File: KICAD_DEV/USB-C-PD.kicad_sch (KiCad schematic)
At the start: 36 parts, among them J1 USB_C_Receptacle_USB2.0_14P, Q1 NMOS, U2 TPS26750, U3 TPD4S480

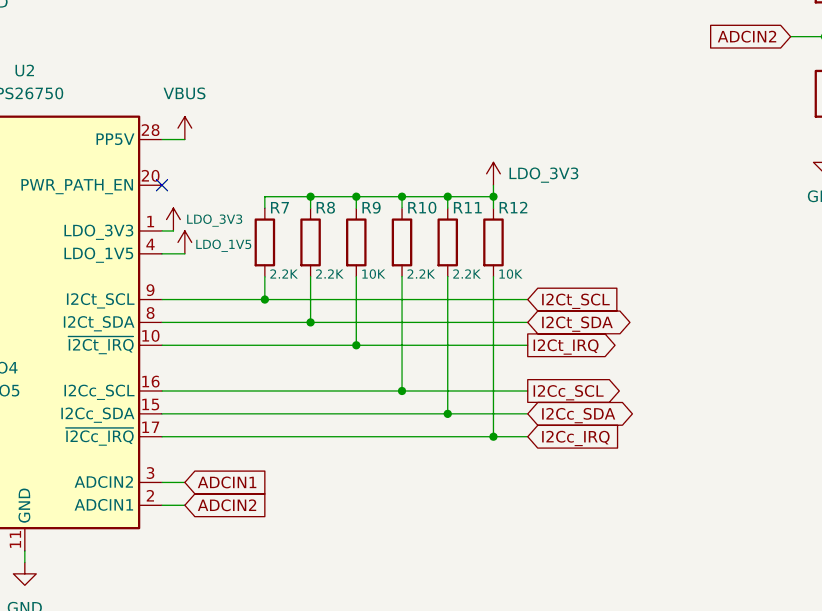
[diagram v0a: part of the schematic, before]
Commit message: updating some stuff
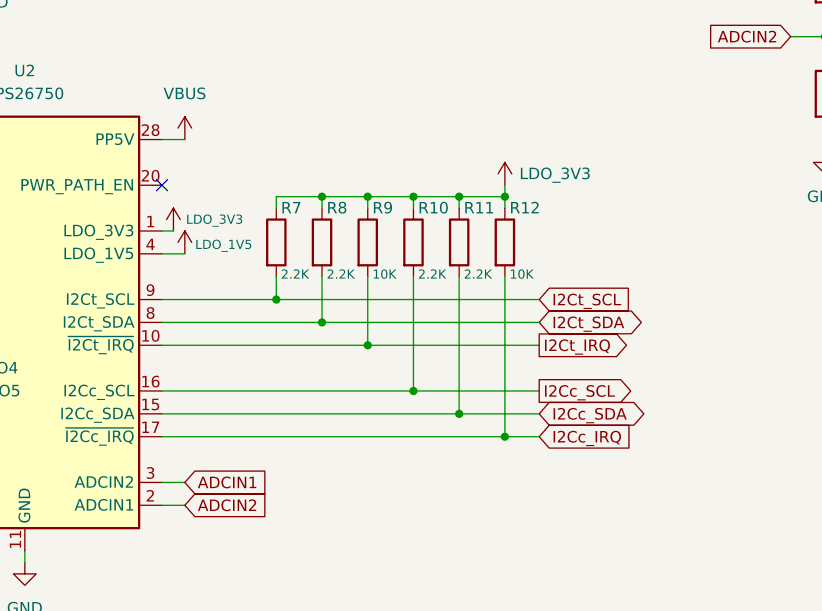
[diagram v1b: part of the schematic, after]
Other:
- moved on the sheet: R10, R11, R12, R7, R8, R9
